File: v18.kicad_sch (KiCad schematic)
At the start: 63 parts, among them U51 ADP5071ACPZ, U52 TPS7A4700xRGW, U53 TPS7A3301RGW

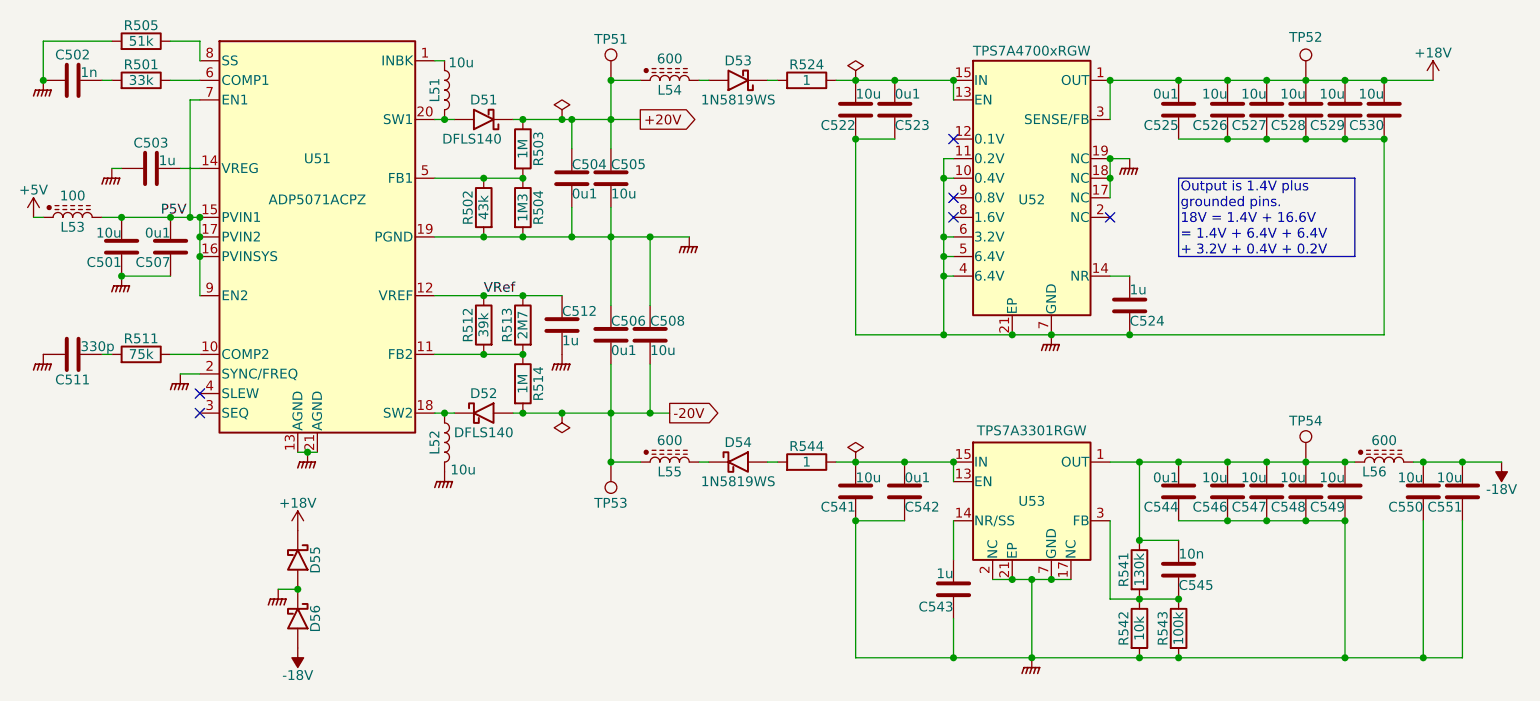
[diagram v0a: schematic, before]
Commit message: Scan deleted.
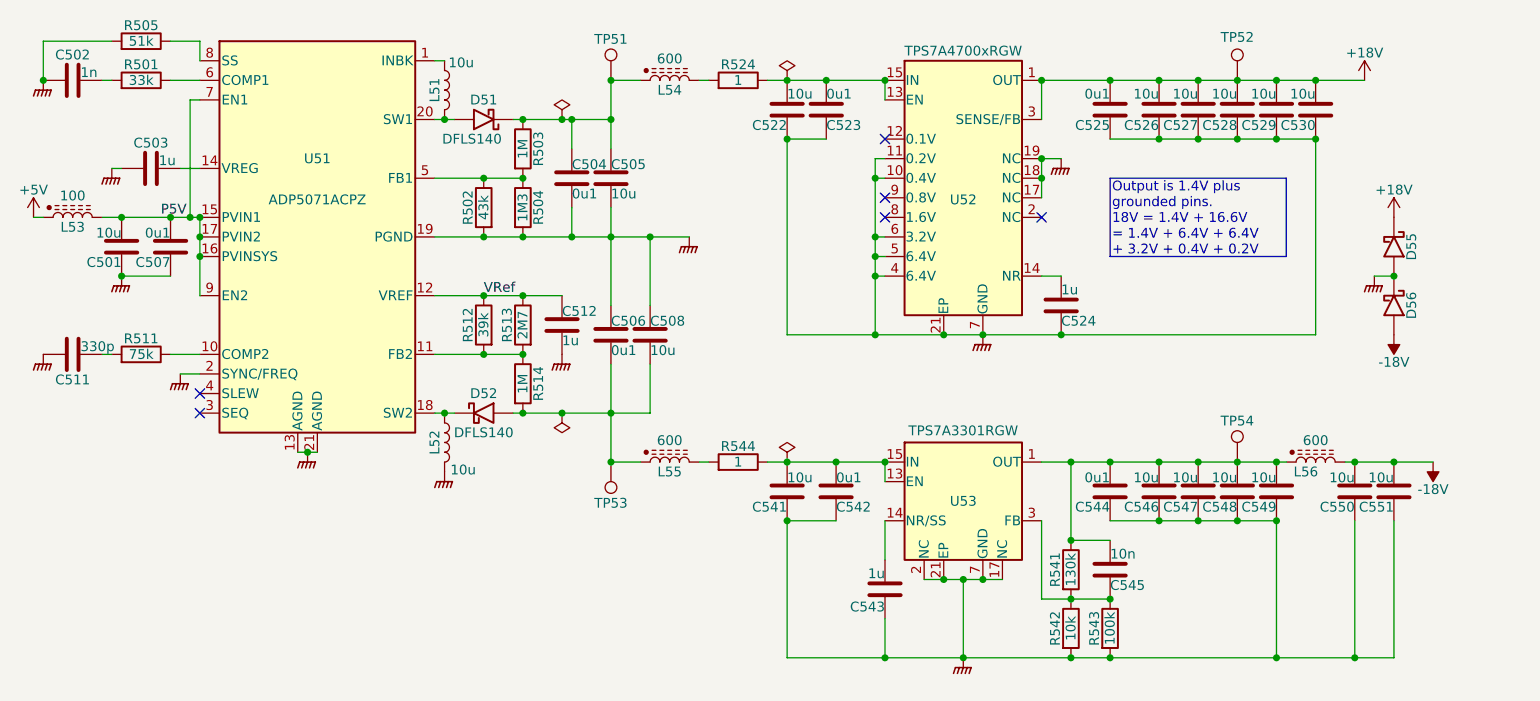
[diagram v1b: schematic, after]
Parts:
- removed D53, D54: 1N5819WS, Diode_SMD:D_SOD-323, symbol Parts:1N5819WS
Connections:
- net at L54.2: now also R524.2
- net at L55.2: now also R544.2
- net +20V: no longer names the net of C504.2, C505.1, D51.1 (K), L54.1, R503.1, TP51.1
- net -20V: no longer names the net of C506.1, C508.2, D52.2 (A), L55.1, R514.2, TP53.1
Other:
- moved on the sheet: C522, C523, C524, C525, C526, C527, C528, C529, C530, C541, C542, C543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

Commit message: Most blocks there....
About to restore scan.
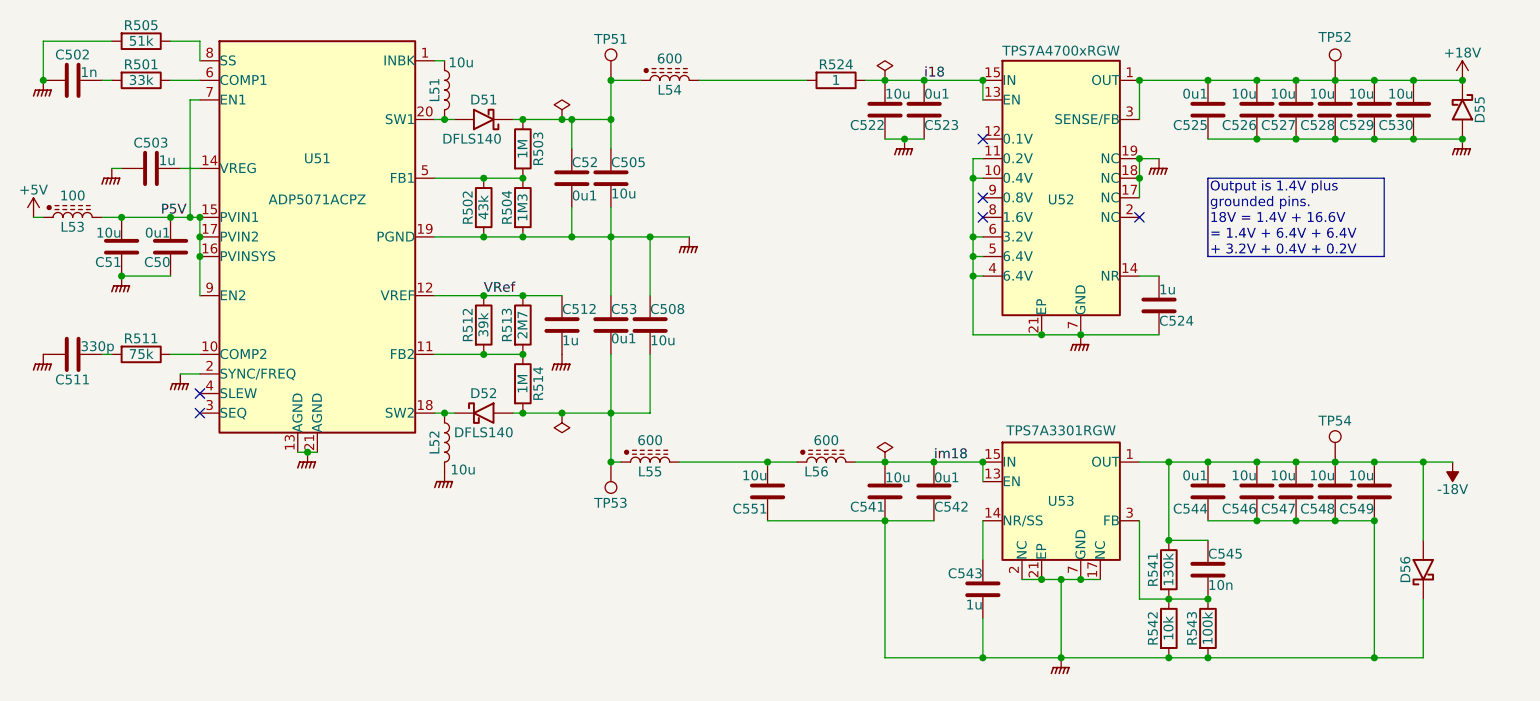
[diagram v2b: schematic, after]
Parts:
- removed C550: 10u, Capacitor_SMD:C_0805_2012Metric, symbol Device:C
- removed R544: 1, Resistor_SMD:R_0603_1608Metric, symbol Device:R
- renumbered C507 to C50, C501 to C51, C504 to C52, C506 to C53
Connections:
- net -18V: now also C544.1, C545.1, C546.1, C547.1, C548.1, C549.1, R541.1, TP54.1, U53.1 (OUT), U53.20 (OUT); no longer C551.2, L56.2
- net GNDPWR: now also C52.2, C522.2, C523.2, C53.1, C543.2, C544.2, C546.2, C547.2, C548.2, C549.2, C551.2; no longer C52.1, C522.1, C523.1, C53.2, C543.1, C544.1, C546.1, C547.1, C548.1, C549.1, C551.1
- net at C505.1, D51.1 (K), L54.1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: now also C52.1; no longer C52.2
- net at C508.2, D52.2 (A), L55.1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: now also C53.2; no longer C53.1
- net i18: now reaches R524.1, U52.13 (EN), U52.15 (IN), U52.16 (IN)
- net i18: now also C522.1, C523.1; no longer C522.2, C523.2
- net at R541.2, R542.1, R543.1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: now also C545.2; no longer C545.1
- net im18: now reaches C541.1, C542.1, U53.13 (EN), U53.15 (IN), U53.16 (IN)
- net im18: now also L56.2
- net at L55.2: now also C551.1, L56.1
- net at U53.14 (NR/SS): now also C543.1; no longer C543.2
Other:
- moved on the sheet: C508, C52, C522, C523, C524, C525, C526, C527, C528, C529, C53, C530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
